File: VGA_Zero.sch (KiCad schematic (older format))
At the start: 31 parts, among them J1 VGA, J19 BARREL_JACK, J2 CONN_02X20, J3 AUDIO, J4 SPI

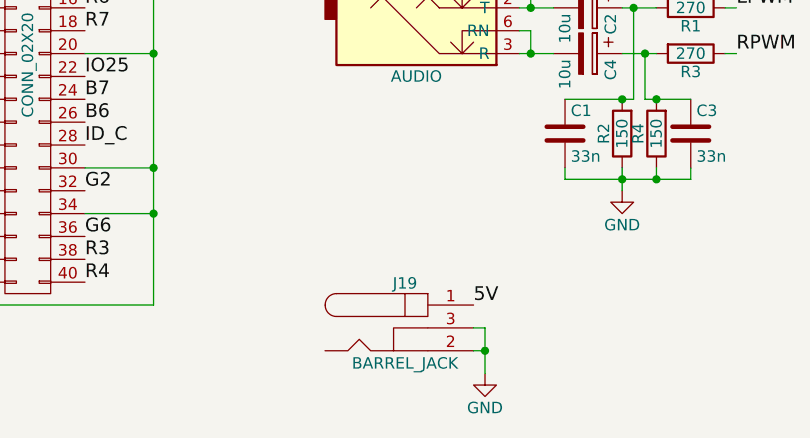
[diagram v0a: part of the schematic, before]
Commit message: rev2
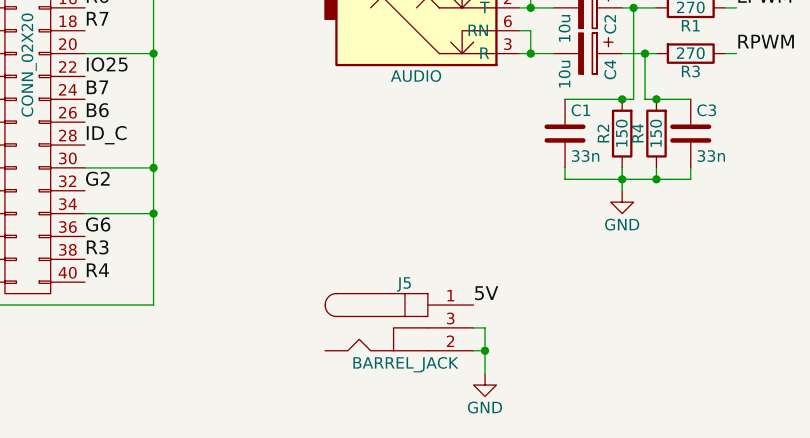
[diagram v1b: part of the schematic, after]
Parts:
- renumbered J19 to J5
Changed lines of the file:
@@
 $EndComp
 $Comp
-L BARREL_JACK J19
+L BARREL_JACK J5
 U 1 1 5992346C
 P 5250 3100
-F 0 "J19" H 5250 3295 50  0000 C CNN
+F 0 "J5" H 5250 3295 50  0000 C CNN
 F 1 "BARREL_JACK" H 5250 2945 50  0000 C CNN
 F 2 "Connectors:BARREL_JACK" H 5250 3100 50  0001 C CNN

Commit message: rev3
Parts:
- removed J4: SPI, Pin_Headers:Pin_Header_Straight_1x07_Pitch2.54mm, symbol CONN_01X07
- added J4: SPI, Pin_Headers:Pin_Header_Straight_1x08_Pitch2.54mm, symbol Connector_Generic:Conn_01x08
- C1, C3: symbol C -> Device:C
- C2, C4: symbol CP -> Device:CP
- J1: symbol DB15_FEMALE_HighDensity -> VGA_Zero-rescue:DB15_FEMALE_HighDensity
- J2: symbol CONN_02X20 -> VGA_Zero-rescue:CONN_02X20
- J3: symbol JACK_TRS_6PINS -> VGA_Zero-rescue:JACK_TRS_6PINS
- J5: symbol BARREL_JACK -> VGA_Zero-rescue:BARREL_JACK
- R1, R2, R3, R4, R5, R6, RB3, RB4, RB5, RB6, RB7, RG2, RG3, RG4, RG5, RG6, RG7, RR3, RR4, RR5, RR6, RR7: symbol R -> Device:R
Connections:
- wire segments 86 -> 121

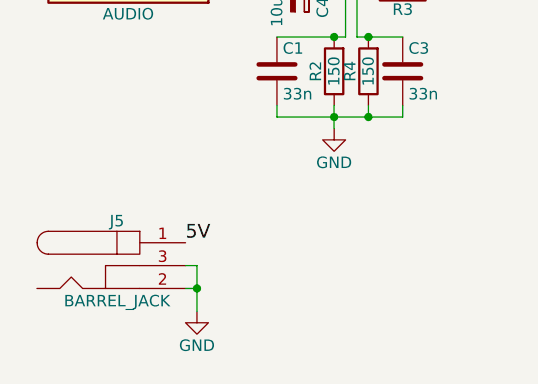
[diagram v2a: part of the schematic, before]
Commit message: rev3
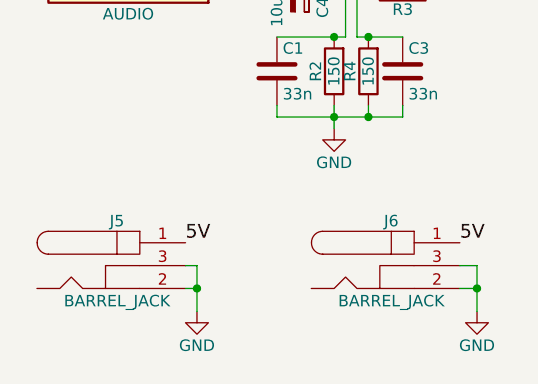
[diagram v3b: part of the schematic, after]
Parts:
- added J6: BARREL_JACK, _LaurentPerso:DC002_3.5x1.1, symbol VGA_Zero-rescue:BARREL_JACK
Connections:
- wire segments 121 -> 125
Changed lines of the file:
@@
 Text Label 1300 2550 0    60   ~ 0
 IO25
+$Comp
+L VGA_Zero-rescue:BARREL_JACK J6
+U 1 1 5C5A2885
+P 6450 3100
+F 0 "J6" H 6450 3295 50  0000 C CNN
+F 1 "BARREL_JACK" H 6450 2945 50  0000 C CNN
+F 2 "_LaurentPerso:DC002_3.5x1.1" H 6450 3100 50  0001 C CNN
+F 3 "" H 6450 3100 50  0001 C CNN
+	1    6450 3100
+	1    0    0    -1
+$EndComp
+Text Label 6750 3000 0    60   ~ 0
+5V
+$Comp
+L power:GND #PWR?
+U 1 1 5C5A2A0D
+P 6825 3300
+F 0 "#PWR?" H 6825 3050 50  0001 C CNN
+F 1 "GND" H 6825 3150 50  0000 C CNN
+F 2 "" H 6825 3300 50  0001 C CNN
+F 3 "" H 6825 3300 50  0001 C CNN
+	1    6825 3300
+	1    0    0    -1
+$EndComp
+Wire Wire Line
+	6750 3100 6825 3100
+Wire Wire Line
+	6825 3100 6825 3200
+Wire Wire Line
+	6750 3200 6825 3200
+Connection ~ 6825 3200
+Wire Wire Line
+	6825 3200 6825 3300
 $EndSCHEMATC

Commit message: Kicad v5.0.2 lib
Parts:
- J1: symbol VGA_Zero-rescue:DB15_FEMALE_HighDensity -> Connector:DB15_Female_HighDensity
- J2: symbol VGA_Zero-rescue:CONN_02X20 -> Connector_Generic:Conn_02x20_Odd_Even
- J3: symbol VGA_Zero-rescue:JACK_TRS_6PINS -> Connector:AudioJack3
- J5, J6: symbol VGA_Zero-rescue:BARREL_JACK -> Connector:Barrel_Jack_Switch
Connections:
- wire segments 125 -> 122
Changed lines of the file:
@@
 $EndDescr
 $Comp
-L VGA_Zero-rescue:CONN_02X20 J2
+L Connector_Generic:Conn_02x20_Odd_Even J2
 U 1 1 597F9289
-P 3600 1950
-F 0 "J2" H 3600 3000 50  0000 C CNN
-F 1 "CONN_02X20" V 3600 1950 50  0000 C CNN
-F 2 "_LaurentPerso:RaspberryPiZeroHAT" H 3600 1000 50  0001 C CNN
-F 3 "" H 3600 1000 50  0001 C CNN
-	1    3600 1950
-	1    0    0    -1
-$EndComp
-$Comp
-L VGA_Zero-rescue:JACK_TRS_6PINS J3
+P 3550 1900
+F 0 "J2" H 3550 2950 50  0000 C CNN
+F 1 "CONN_02X20" V 3550 1900 50  0000 C CNN
+F 2 "_LaurentPerso:RaspberryPiZeroHAT" H 3550 950 50  0001 C CNN
+F 3 "" H 3550 950 50  0001 C CNN
+	1    3550 1900
+	1    0    0    -1
+$EndComp
+$Comp
+L Connector:AudioJack3 J3
 U 1 1 597FA528
 P 5350 1700
-F 0 "J3" H 5350 2100 50  0000 C CNN
+F 0 "J3" H 5325 1925 50  0000 C CNN
 F 1 "AUDIO" H 5300 1400 50  0000 C CNN
 F 2 "_LaurentPerso:jack3.5smd" H 5450 1550 50  0001 C CNN
@@
 	1    0    0    -1
 $EndComp
-Wire Wire Line
-	5750 1400 5800 1400
-Wire Wire Line
-	5750 1500 5800 1500
-Wire Wire Line
-	5800 1500 5800 1400
-Connection ~ 5800 1400
 $Comp
 L Device:CP C2
@@
 	0    1    1    0
 $EndComp
-Wire Wire Line
-	5900 1700 5800 1700
-Wire Wire Line
-	5900 1900 5800 1900
-Wire Wire Line
-	5750 1800 5800 1800
-Wire Wire Line
-	5800 1800 5800 1900
-Connection ~ 5800 1900
-Wire Wire Line
-	5750 1600 5800 1600
-Wire Wire Line
-	5800 1600 5800 1700
-Connection ~ 5800 1700
 $Comp
 L Device:R R1
@@
 	1650 3150 1650 3200
 $Comp
-L VGA_Zero-rescue:DB15_FEMALE_HighDensity J1
+L Connector:DB15_Female_HighDensity J1
 U 1 1 59848D1D
 P 1450 1350
@@
 $EndComp
 $Comp
-L VGA_Zero-rescue:BARREL_JACK J5
+L Connector:Barrel_Jack_Switch J5
 U 1 1 5992346C
 P 5250 3100
 F 0 "J5" H 5250 3295 50  0000 C CNN
-F 1 "BARREL_JACK" H 5250 2945 50  0000 C CNN
+F 1 "BARREL_JACK" H 5250 2900 50  0000 C CNN
 F 2 "Connectors:BARREL_JACK" H 5250 3100 50  0001 C CNN
 F 3 "" H 5250 3100 50  0001 C CNN
@@
 Wire Wire Line
 	4150 2600 4150 3000
-Wire Wire Line
-	5800 1400 6050 1400
-Wire Wire Line
-	5800 1900 5750 1900
-Wire Wire Line
-	5800 1700 5750 1700
 Wire Wire Line
 	6250 1700 6350 1700
@@
 IO25
 $Comp
-L VGA_Zero-rescue:BARREL_JACK J6
+L Connector:Barrel_Jack_Switch J6
 U 1 1 5C5A2885
 P 6450 3100
 F 0 "J6" H 6450 3295 50  0000 C CNN
-F 1 "BARREL_JACK" H 6450 2945 50  0000 C CNN
+F 1 "BARREL_JACK" H 6450 2900 50  0000 C CNN
 F 2 "_LaurentPerso:DC002_3.5x1.1" H 6450 3100 50  0001 C CNN
 F 3 "" H 6450 3100 50  0001 C CNN
@@
 Wire Wire Line
 	6825 3200 6825 3300
+Wire Wire Line
+	5550 1600 5625 1600
+Wire Wire Line
+	5625 1600 5625 1400
+Wire Wire Line
+	5625 1400 6050 1400
+Wire Wire Line
+	5675 1700 5675 1800
+Wire Wire Line
+	5675 1800 5550 1800
+Wire Wire Line
+	5675 1700 5900 1700
+Wire Wire Line
+	5625 1900 5625 1700
+Wire Wire Line
+	5625 1700 5550 1700
+Wire Wire Line
+	5625 1900 5900 1900
 $EndSCHEMATC
